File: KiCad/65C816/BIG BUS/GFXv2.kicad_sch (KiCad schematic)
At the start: 6 parts, among them J10 Bus Header, U11 6522, U13 320x240 LCD

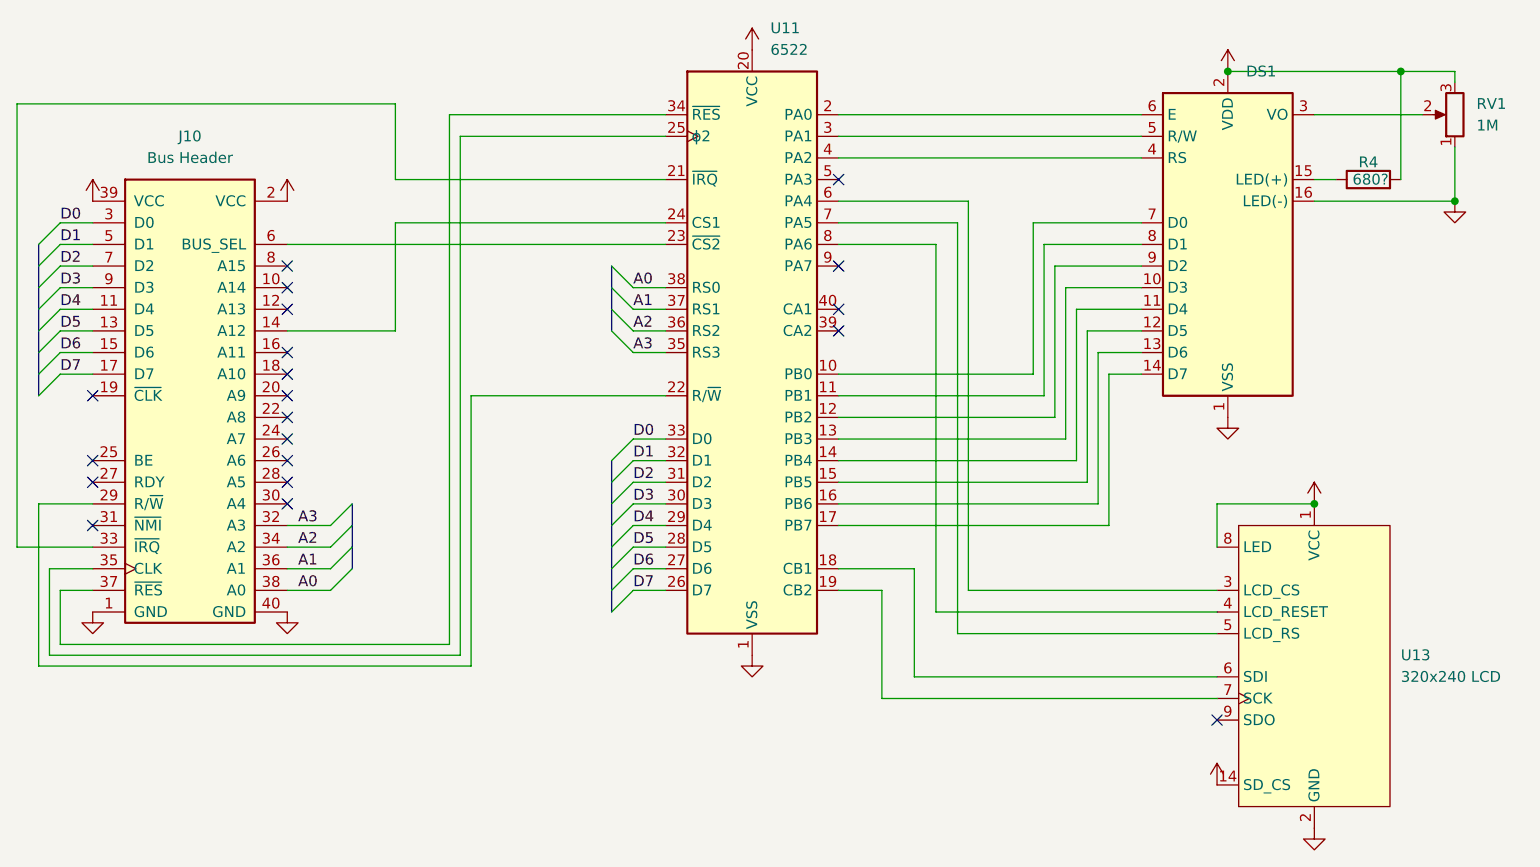
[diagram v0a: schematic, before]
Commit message: Cleaned up random files, added actual .gitignore on my end lmao
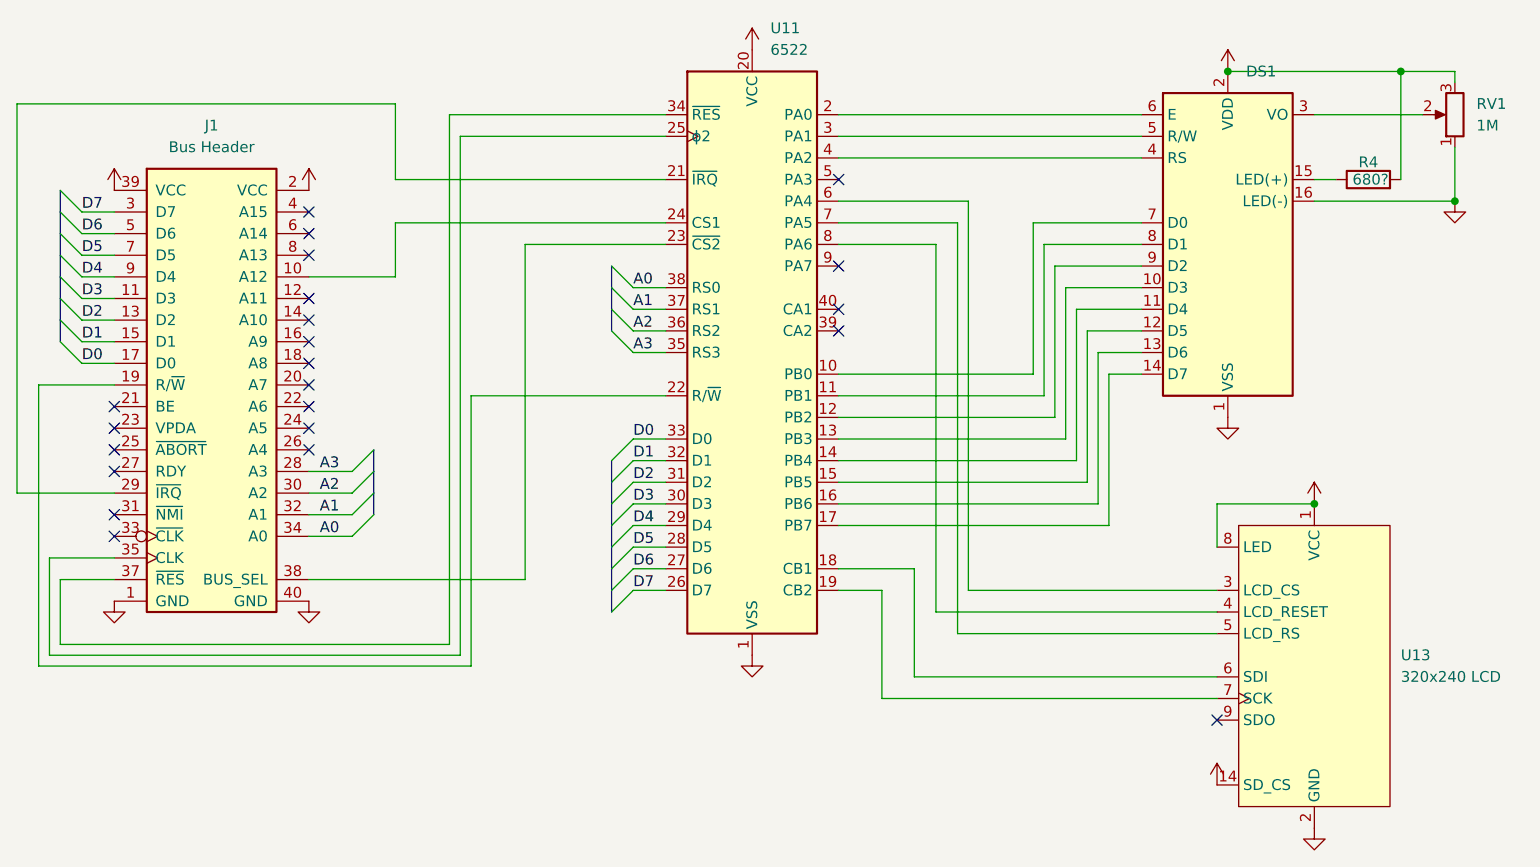
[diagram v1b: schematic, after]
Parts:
- removed J10: Bus Header, Connector_PinHeader_2.54mm:PinHeader_2x20_P2.54mm_Vertical, symbol Board Connectors:Generic Board Connector
- added J1: Bus Header, Connector_IDC:IDC-Header_2x20_P2.54mm_Vertical, symbol Board Connectors:Board_Bus_V2
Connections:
- net +5V: now also J1.2 (VCC), J1.39 (VCC)
- net A0: now also J1.34 (A0)
- net A1: now also J1.32 (A1)
- net A2: now also J1.30 (A2)
- net A3: now also J1.28 (A3)
- net D0: now also J1.17 (D0)
- net D1: now also J1.15 (D1)
- net D2: now also J1.13 (D2)
- net D3: now also J1.11 (D3)
- net D4: now also J1.9 (D4)
- net D5: now also J1.7 (D5)
- net D6: now also J1.5 (D6)
- net D7: now also J1.3 (D7)
- net GND: now also J1.1 (GND), J1.40 (GND)
- net at U11.21 (~{IRQ}): now also J1.29 (~{IRQ})
- net at U11.22 (R/~{W}): now also J1.19 (R/~{W})
- net at U11.23 (~{CS2}): now also J1.38 (BUS_SEL)
- net at U11.24 (CS1): now also J1.10 (A12)
- net at U11.25 (ϕ2): now also J1.35 (CLK)
- net at U11.34 (~{RES}): now also J1.37 (~{RES})
- no-connect marks 20 -> 22
